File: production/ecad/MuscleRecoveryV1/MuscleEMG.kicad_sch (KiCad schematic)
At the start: 42 parts, among them J1 AudioJack3, J2 Screw_Terminal_01x03, J8 Screw_Terminal_01x07, U5 AD8232ACPZ-R7, U7 ADS1115IDGS

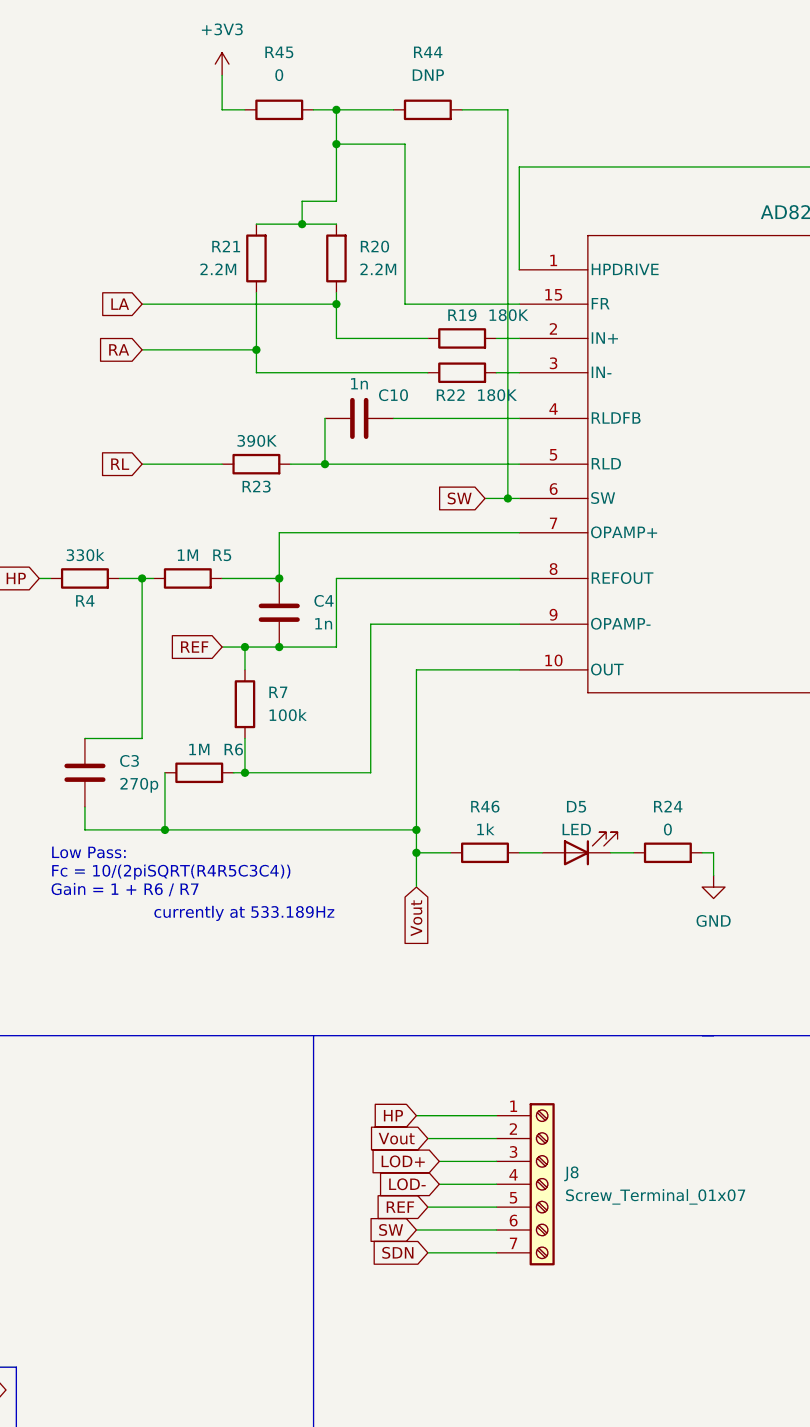
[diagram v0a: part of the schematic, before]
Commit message: saving changes
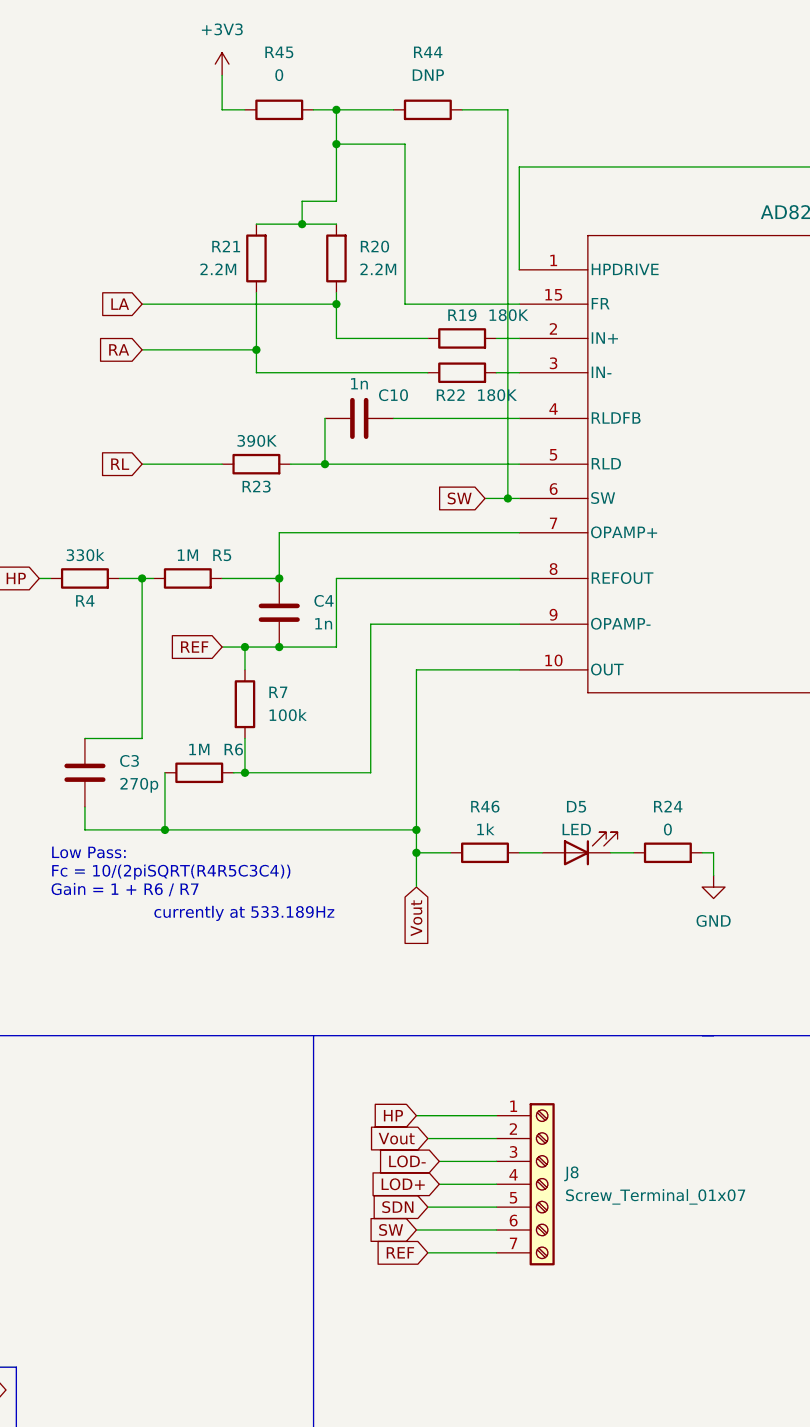
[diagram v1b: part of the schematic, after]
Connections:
- net LOD+: now also J8.4 (Pin_4); no longer J8.3 (Pin_3)
- net LOD-: now also J8.3 (Pin_3); no longer J8.4 (Pin_4)
- net REF: now also J8.7 (Pin_7); no longer J8.5 (Pin_5)
- net SDN: now also J8.5 (Pin_5); no longer J8.7 (Pin_7)
- net SW: now also R44.1; no longer R44.2
- net at R20.2, R21.2, R45.2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: now also R44.2; no longer R44.1
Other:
- moved on the sheet: R44
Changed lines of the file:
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@@
     )
   )
-  (global_label "LOD-" (shape input) (at 139.7 142.24 180) (fields_autoplaced)
+  (global_label "LOD-" (shape input) (at 139.7 139.7 180) (fields_autoplaced)
+    (effects (font (size 1.27 1.27)) (justify right))
+    (property "Intersheetrefs" "${INTERSHEET_REFS}" (at 131.5138 139.7 0)
+      (effects (font (size 1.27 1.27)) (justify right) hide)
+    )
+  )
+  (global_label "SW" (shape input) (at 144.78 66.04 180) (fields_autoplaced)
+    (effects (font (size 1.27 1.27)) (justify right))
+    (property "Intersheetrefs" "${INTERSHEET_REFS}" (at 139.1339 66.04 0)
+      (effects (font (size 1.27 1.27)) (justify right) hide)
+    )
+  )
+  (global_label "LA" (shape input) (at 106.68 44.45 180) (fields_autoplaced)
+    (effects (font (size 1.27 1.27)) (justify right))
+    (property "Intersheetrefs" "${INTERSHEET_REFS}" (at 101.5781 44.45 0)
+      (effects (font (size 1.27 1.27)) (justify right) hide)
+    )
+  )
+  (global_label "HP" (shape input) (at 95.25 74.93 180) (fields_autoplaced)
+    (effects (font (size 1.27 1.27)) (justify right))
+    (property "Intersheetrefs" "${INTERSHEET_REFS}" (at 89.6643 74.93 0)
+      (effects (font (size 1.27 1.27)) (justify right) hide)
+    )
+  )
+  (global_label "RL" (shape input) (at 106.68 62.23 180) (fields_autoplaced)
+    (effects (font (size 1.27 1.27)) (justify right))
+    (property "Intersheetrefs" "${INTERSHEET_REFS}" (at 101.3967 62.23 0)
+      (effects (font (size 1.27 1.27)) (justify right) hide)
+    )
+  )
+  (global_label "Vout" (shape input) (at 137.16 109.22 270) (fields_autoplaced)
+    (effects (font (size 1.27 1.27)) (justify right))
+    (property "Intersheetrefs" "${INTERSHEET_REFS}" (at 137.16 116.3175 90)
+      (effects (font (size 1.27 1.27)) (justify right) hide)
+    )
+  )
+  (global_label "LOD+" (shape input) (at 139.7 142.24 180) (fields_autoplaced)
     (effects (font (size 1.27 1.27)) (justify right))
     (property "Intersheetrefs" "${INTERSHEET_REFS}" (at 131.5138 142.24 0)
@@
     )
   )
-  (global_label "SW" (shape input) (at 144.78 66.04 180) (fields_autoplaced)
-    (effects (font (size 1.27 1.27)) (justify right))
-    (property "Intersheetrefs" "${INTERSHEET_REFS}" (at 139.1339 66.04 0)
-      (effects (font (size 1.27 1.27)) (justify right) hide)
-    )
-  )
-  (global_label "LA" (shape input) (at 106.68 44.45 180) (fields_autoplaced)
-    (effects (font (size 1.27 1.27)) (justify right))
-    (property "Intersheetrefs" "${INTERSHEET_REFS}" (at 101.5781 44.45 0)
-      (effects (font (size 1.27 1.27)) (justify right) hide)
-    )
-  )
-  (global_label "HP" (shape input) (at 95.25 74.93 180) (fields_autoplaced)
-    (effects (font (size 1.27 1.27)) (justify right))
-    (property "Intersheetrefs" "${INTERSHEET_REFS}" (at 89.6643 74.93 0)
-      (effects (font (size 1.27 1.27)) (justify right) hide)
-    )
-  )
-  (global_label "RL" (shape input) (at 106.68 62.23 180) (fields_autoplaced)
-    (effects (font (size 1.27 1.27)) (justify right))
-    (property "Intersheetrefs" "${INTERSHEET_REFS}" (at 101.3967 62.23 0)
-      (effects (font (size 1.27 1.27)) (justify right) hide)
-    )
-  )
-  (global_label "REF" (shape input) (at 138.43 144.78 180) (fields_autoplaced)
-    (effects (font (size 1.27 1.27)) (justify right))
-    (property "Intersheetrefs" "${INTERSHEET_REFS}" (at 131.9372 144.78 0)
-      (effects (font (size 1.27 1.27)) (justify right) hide)
-    )
-  )
-  (global_label "Vout" (shape input) (at 137.16 109.22 270) (fields_autoplaced)
-    (effects (font (size 1.27 1.27)) (justify right))
-    (property "Intersheetrefs" "${INTERSHEET_REFS}" (at 137.16 116.3175 90)
-      (effects (font (size 1.27 1.27)) (justify right) hide)
-    )
-  )
   (global_label "REF" (shape input) (at 115.57 82.55 180) (fields_autoplaced)
     (effects (font (size 1.27 1.27)) (justify right))
@@
     )
   )
+  (global_label "REF" (shape input) (at 138.43 149.86 180) (fields_autoplaced)
+    (effects (font (size 1.27 1.27)) (justify right))
+    (property "Intersheetrefs" "${INTERSHEET_REFS}" (at 131.9372 149.86 0)
+      (effects (font (size 1.27 1.27)) (justify right) hide)
+    )
+  )
   (global_label "RL" (shape input) (at 35.56 66.04 0) (fields_autoplaced)
     (effects (font (size 1.27 1.27)) (justify left))
@@
     )
   )
-  (global_label "LOD+" (shape input) (at 139.7 139.7 180) (fields_autoplaced)
-    (effects (font (size 1.27 1.27)) (justify right))
-    (property "Intersheetrefs" "${INTERSHEET_REFS}" (at 131.5138 139.7 0)
-      (effects (font (size 1.27 1.27)) (justify right) hide)
-    )
-  )
   (global_label "LA" (shape input) (at 35.56 63.5 0) (fields_autoplaced)
     (effects (font (size 1.27 1.27)) (justify left))
@@
     )
   )
-  (global_label "SDN" (shape input) (at 138.43 149.86 180) (fields_autoplaced)
-    (effects (font (size 1.27 1.27)) (justify right))
-    (property "Intersheetrefs" "${INTERSHEET_REFS}" (at 131.6348 149.86 0)
-      (effects (font (size 1.27 1.27)) (justify right) hide)
-    )
-  )
   (global_label "RL" (shape input) (at 41.91 96.52 0) (fields_autoplaced)
     (effects (font (size 1.27 1.27)) (justify left))
@@
     (property "Intersheetrefs" "${INTERSHEET_REFS}" (at 226.5052 77.47 0)
       (effects (font (size 1.27 1.27)) (justify left) hide)
+    )
+  )
+  (global_label "SDN" (shape input) (at 138.43 144.78 180) (fields_autoplaced)
+    (effects (font (size 1.27 1.27)) (justify right))
+    (property "Intersheetrefs" "${INTERSHEET_REFS}" (at 131.6348 144.78 0)
+      (effects (font (size 1.27 1.27)) (justify right) hide)
     )
   )
@@
     )
   )
-  (symbol (lib_id "Device:R") (at 138.43 22.86 90) (unit 1)
-    (in_bom yes) (on_board yes) (dnp no) (fields_autoplaced)
+  (symbol (lib_id "Device:R") (at 138.43 22.86 270) (mirror x) (unit 1)
+    (in_bom yes) (on_board yes) (dnp no)
     (property "Reference" "R44" (at 138.43 16.51 90)
       (effects (font (size 1.27 1.27)))
